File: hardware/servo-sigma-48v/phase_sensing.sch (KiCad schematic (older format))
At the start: 31 parts, among them U10 OPA4374, U9 OPA4374

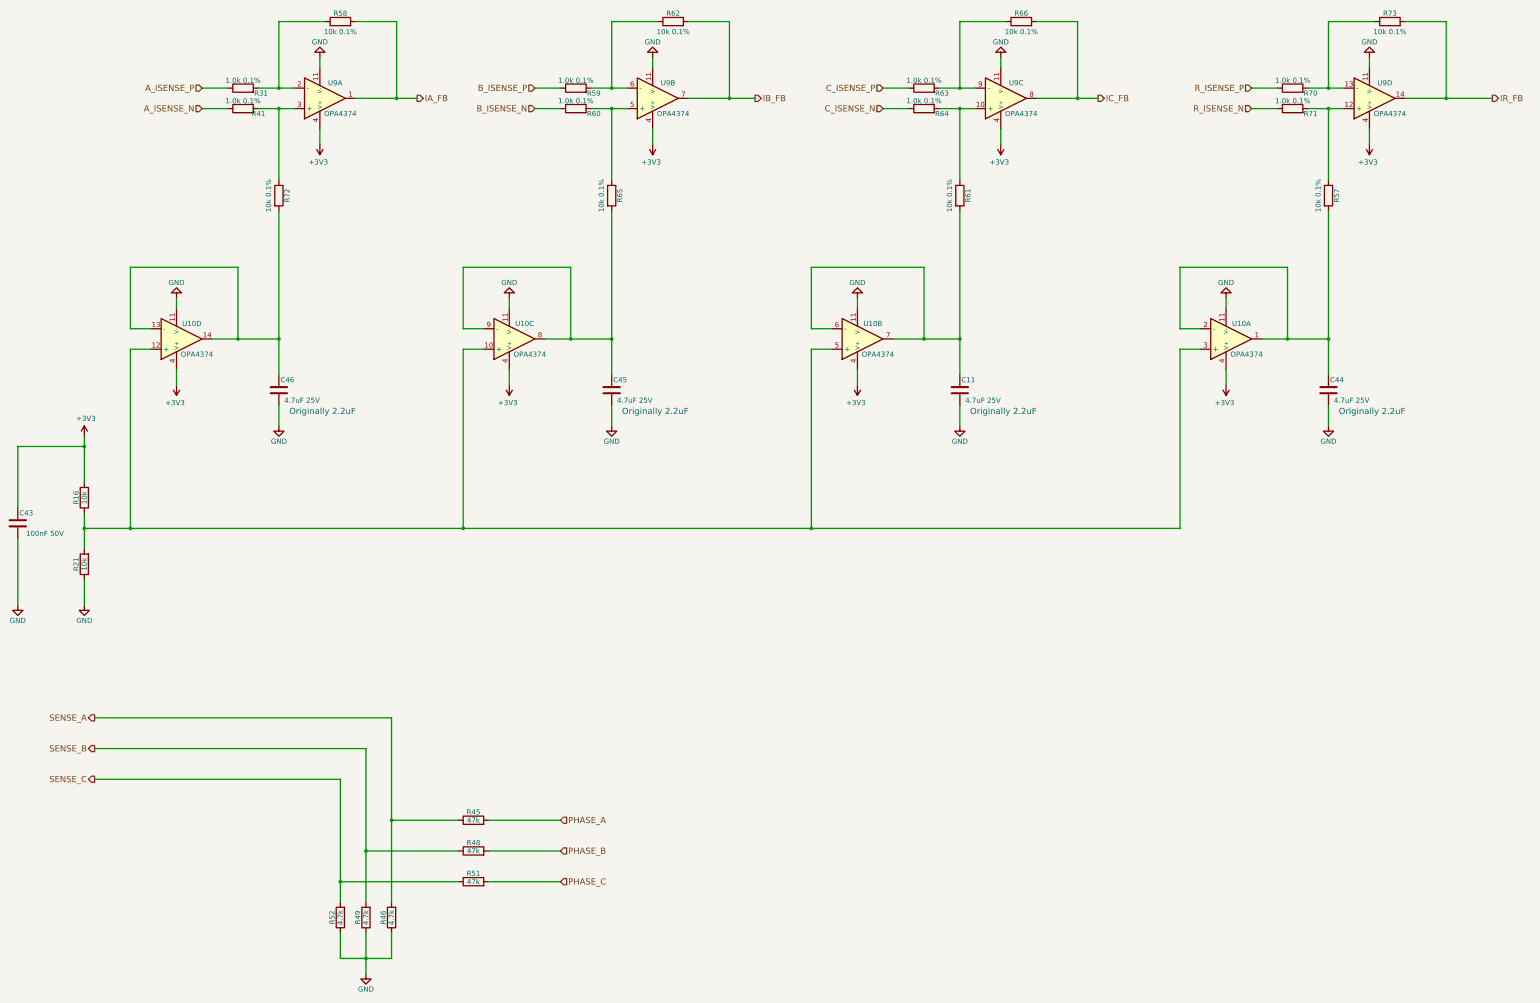
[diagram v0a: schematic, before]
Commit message: work on rs485
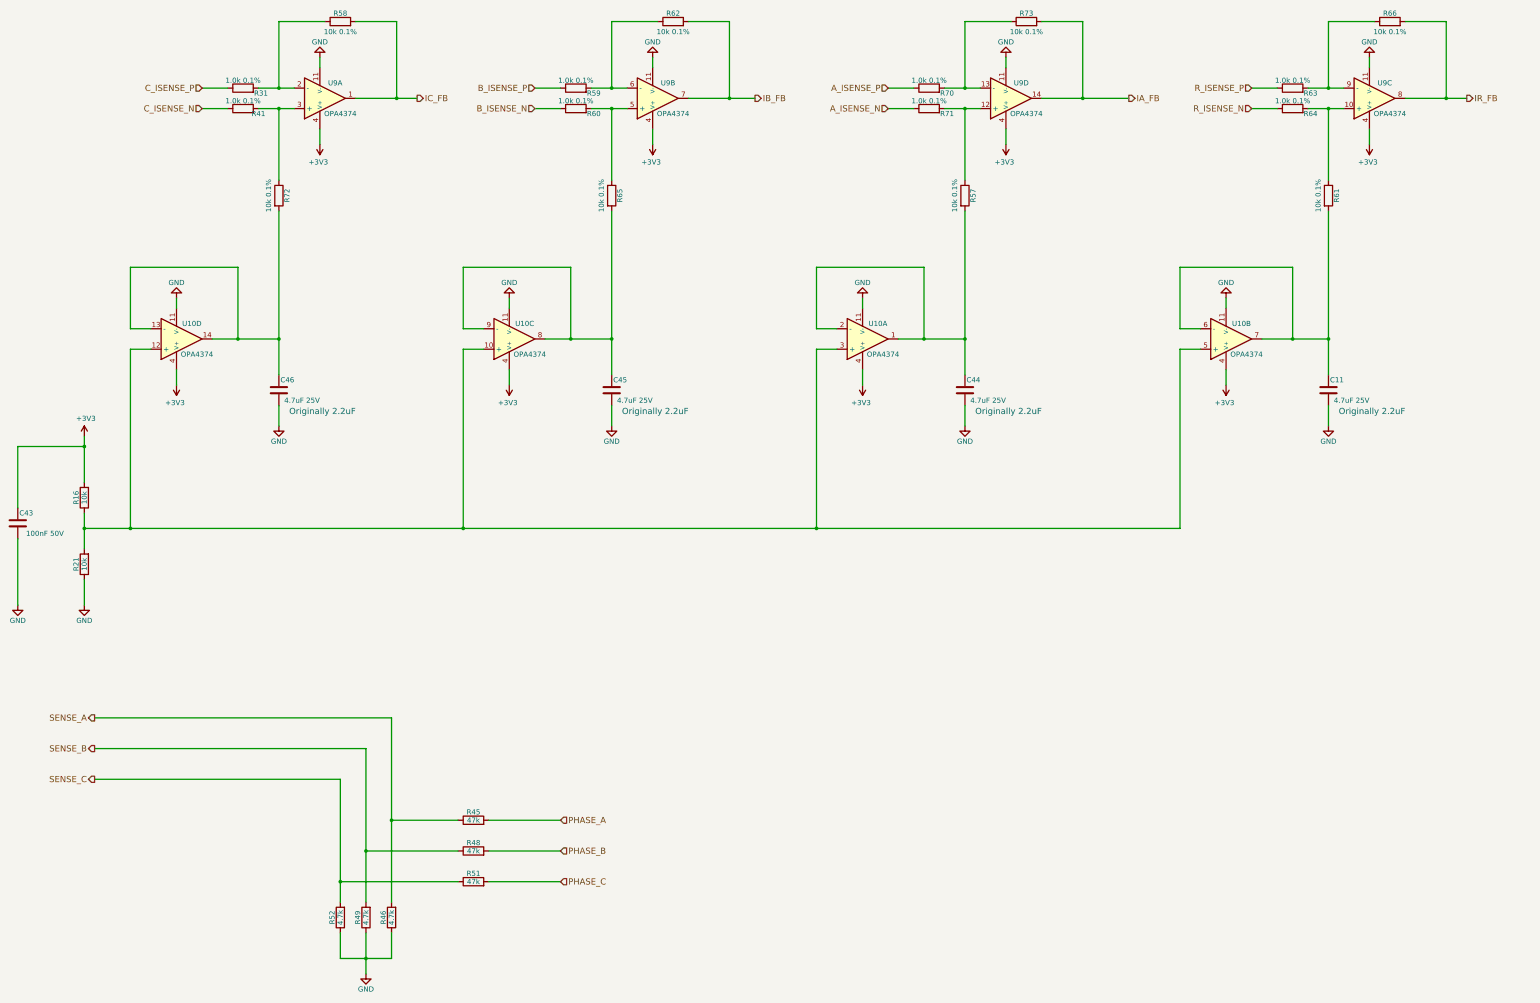
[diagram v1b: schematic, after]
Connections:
- net A_ISENSE_N: now also R71.1; no longer R41.1
- net A_ISENSE_P: now also R70.1; no longer R31.1
- net C_ISENSE_N: now also R41.1; no longer R64.1
- net C_ISENSE_P: now also R31.1; no longer R63.1
- net IA_FB: now also R73.2, U9.14; no longer R58.2, U9.1
- net IC_FB: now also R58.2, U9.1; no longer R66.2, U9.8
- net IR_FB: now also R66.2, U9.8; no longer R73.2, U9.14
- net R_ISENSE_N: now also R64.1; no longer R71.1
- net R_ISENSE_P: now also R63.1; no longer R70.1
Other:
- moved on the sheet: C11, C44, R57, R61, R63, R64, R66, R70, R71, R73, U10A, U10B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
